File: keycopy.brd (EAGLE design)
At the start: 102.2 x 38.1 mm, 86 parts

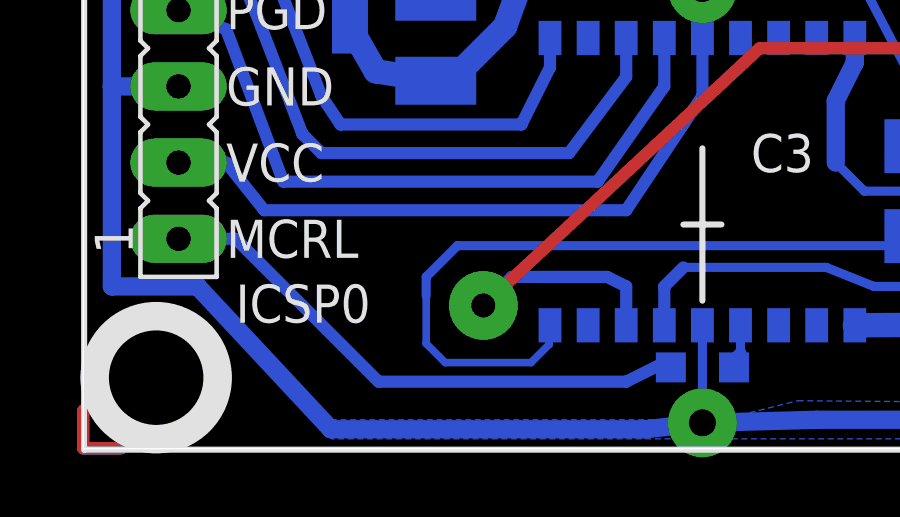
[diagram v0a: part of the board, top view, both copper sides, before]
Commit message: 2016.07.05
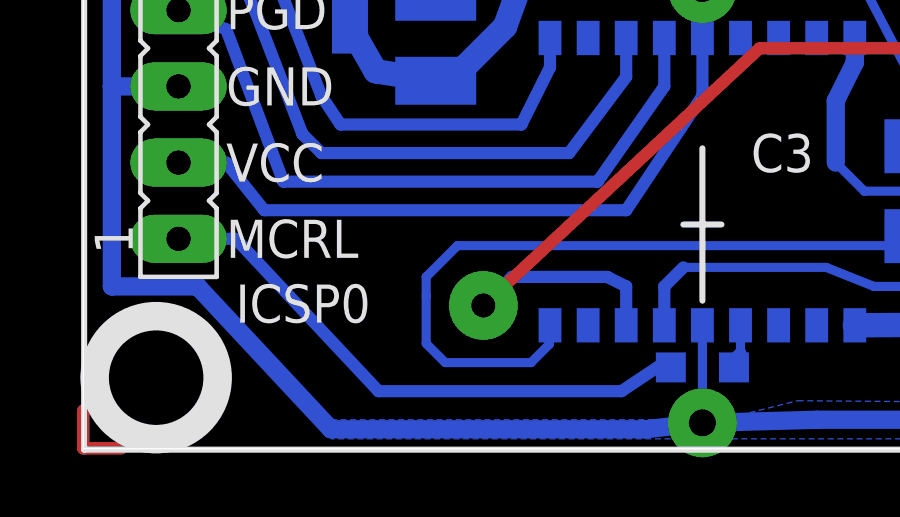
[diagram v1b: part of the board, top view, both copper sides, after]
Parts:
- L3: value 100uH -> 30uH
- R24: value 3k -> (3k&22k)
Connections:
- net N$5 renamed 1W_
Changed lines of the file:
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@@
 <setting verticaltext="up"/>
 </settings>
-<grid distance="12.5" unitdist="mil" unit="mil" style="lines" multiple="1" display="yes" altdistance="0.025" altunitdist="inch" altunit="inch"/>
+<grid distance="50" unitdist="mil" unit="mil" style="lines" multiple="1" display="yes" altdistance="0.025" altunitdist="inch" altunit="inch"/>
 <layers>
 <layer number="1" name="Top" color="4" fill="1" visible="yes" active="yes"/>
@@
 <attribute name="VALUE" x="13.462" y="15.494" size="1.27" layer="28" rot="MR0"/>
 </element>
-<element name="R24" library="resistor" package="R1206W" value="3k" x="9.525" y="16.1925" smashed="yes" rot="MR270">
+<element name="R24" library="resistor" package="R1206W" value="(3k&amp;22k)" x="9.525" y="16.1925" smashed="yes" rot="MR270">
 <attribute name="NAME" x="8.4455" y="10.7315" size="1.27" layer="26" rot="MR90"/>
 <attribute name="VALUE" x="11.938" y="17.8435" size="1.27" layer="28" rot="MR270"/>
@@
 <attribute name="VALUE" x="54.099165625" y="25.9108375" size="0.02" layer="28" rot="MR225"/>
 </element>
-<element name="L3" library="rcl" package="0207/12" value="100uH" x="26.9875" y="19.05" smashed="yes">
+<element name="L3" library="rcl" package="0207/12" value="30uH" x="26.9875" y="19.05" smashed="yes">
 <attribute name="NAME" x="25.7175" y="18.2245" size="1.27" layer="25" ratio="10"/>
 <attribute name="VALUE" x="24.7015" y="18.3642" size="1.27" layer="27" ratio="10"/>
@@
 <wire x1="13.106" y1="7.391" x2="27.6225" y2="7.391" width="0.3048" layer="16"/>
 <wire x1="27.6225" y1="7.391" x2="27.94" y2="7.7085" width="0.3048" layer="16"/>
-<wire x1="16.1671" y1="4.7625" x2="16.1671" y2="4.1021" width="0.254" layer="16"/>
-<wire x1="16.1671" y1="4.1021" x2="15.5575" y2="3.4925" width="0.254" layer="16"/>
-<wire x1="15.5575" y1="3.4925" x2="12.7" y2="3.4925" width="0.254" layer="16"/>
-<wire x1="12.7" y1="3.4925" x2="12.065" y2="4.1275" width="0.254" layer="16"/>
-<wire x1="12.065" y1="4.1275" x2="12.065" y2="5.715" width="0.254" layer="16"/>
+<wire x1="16.1671" y1="4.7625" x2="16.1671" y2="4.1021" width="0.3048" layer="16"/>
+<wire x1="16.1671" y1="4.1021" x2="15.5575" y2="3.4925" width="0.3048" layer="16"/>
+<wire x1="15.5575" y1="3.4925" x2="12.7" y2="3.4925" width="0.3048" layer="16"/>
+<wire x1="12.7" y1="3.4925" x2="12.065" y2="4.1275" width="0.3048" layer="16"/>
+<wire x1="12.065" y1="4.1275" x2="12.065" y2="5.715" width="0.3048" layer="16"/>
 </signal>
 <signal name="PGM">
@@
 <wire x1="79.375" y1="18.0975" x2="75.565" y2="19.3675" width="0.4064" layer="16"/>
 </signal>
-<signal name="N$5">
+<signal name="1W_">
 <contactref element="DD1" pad="6"/>
 <via x="30.1625" y="6.6675" extent="1-16" drill="0.8" diameter="2.3"/>
@@
 <wire x1="5.715" y1="7.62" x2="3.81" y2="7.62" width="0.4064" layer="16"/>
 <wire x1="20.22" y1="3.33375" x2="20.0025" y2="3.4925" width="0.4064" layer="16"/>
-<wire x1="20.0025" y1="3.4925" x2="18.7325" y2="2.8575" width="0.4064" layer="16"/>
-<wire x1="18.7325" y1="2.8575" x2="10.4775" y2="2.8575" width="0.4064" layer="16"/>
-<wire x1="10.4775" y1="2.8575" x2="5.715" y2="7.62" width="0.4064" layer="16"/>
+<wire x1="20.0025" y1="3.4925" x2="18.57375" y2="2.54" width="0.4064" layer="16"/>
+<wire x1="18.57375" y1="2.54" x2="10.4775" y2="2.54" width="0.4064" layer="16"/>
+<wire x1="10.4775" y1="2.54" x2="5.715" y2="7.62" width="0.4064" layer="16"/>
 </signal>
 <signal name="N$25">
